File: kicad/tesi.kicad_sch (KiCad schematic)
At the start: 35 parts, among them J1 Conn_01x03_Pin, J2 Conn_01x03_Pin, J3 Conn_01x04_Pin, J4 Conn_01x02_Pin, SW1 POWER, U1 MAX4466, U2 BNO055, U3 MPR121, U4 VL53L1CX

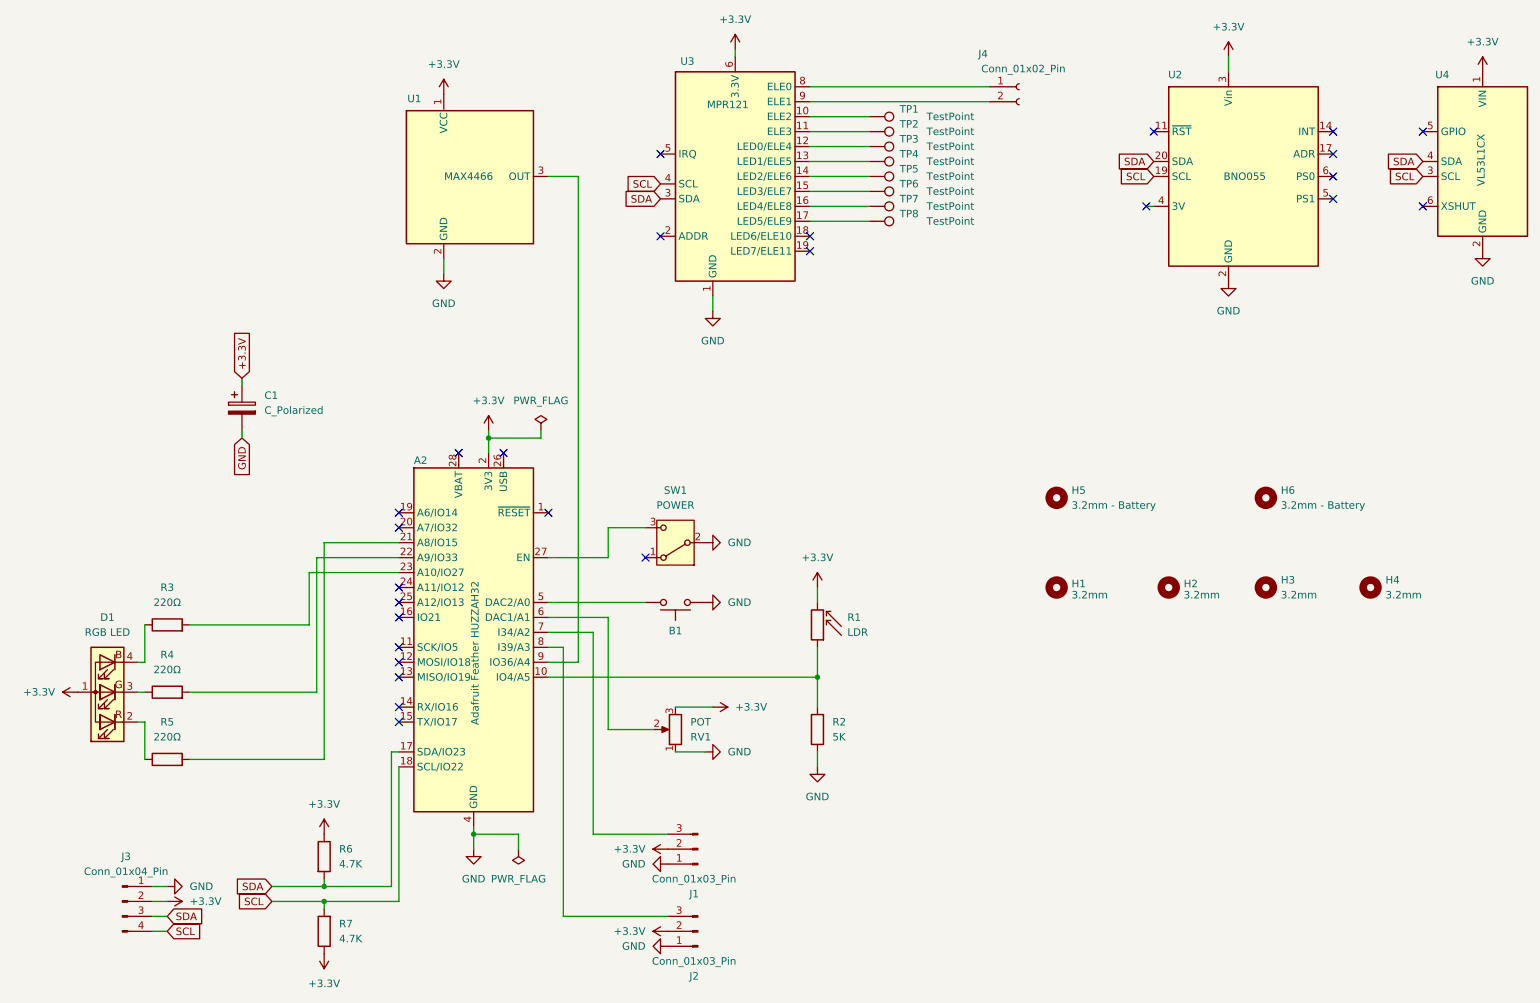
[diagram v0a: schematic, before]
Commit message: updates
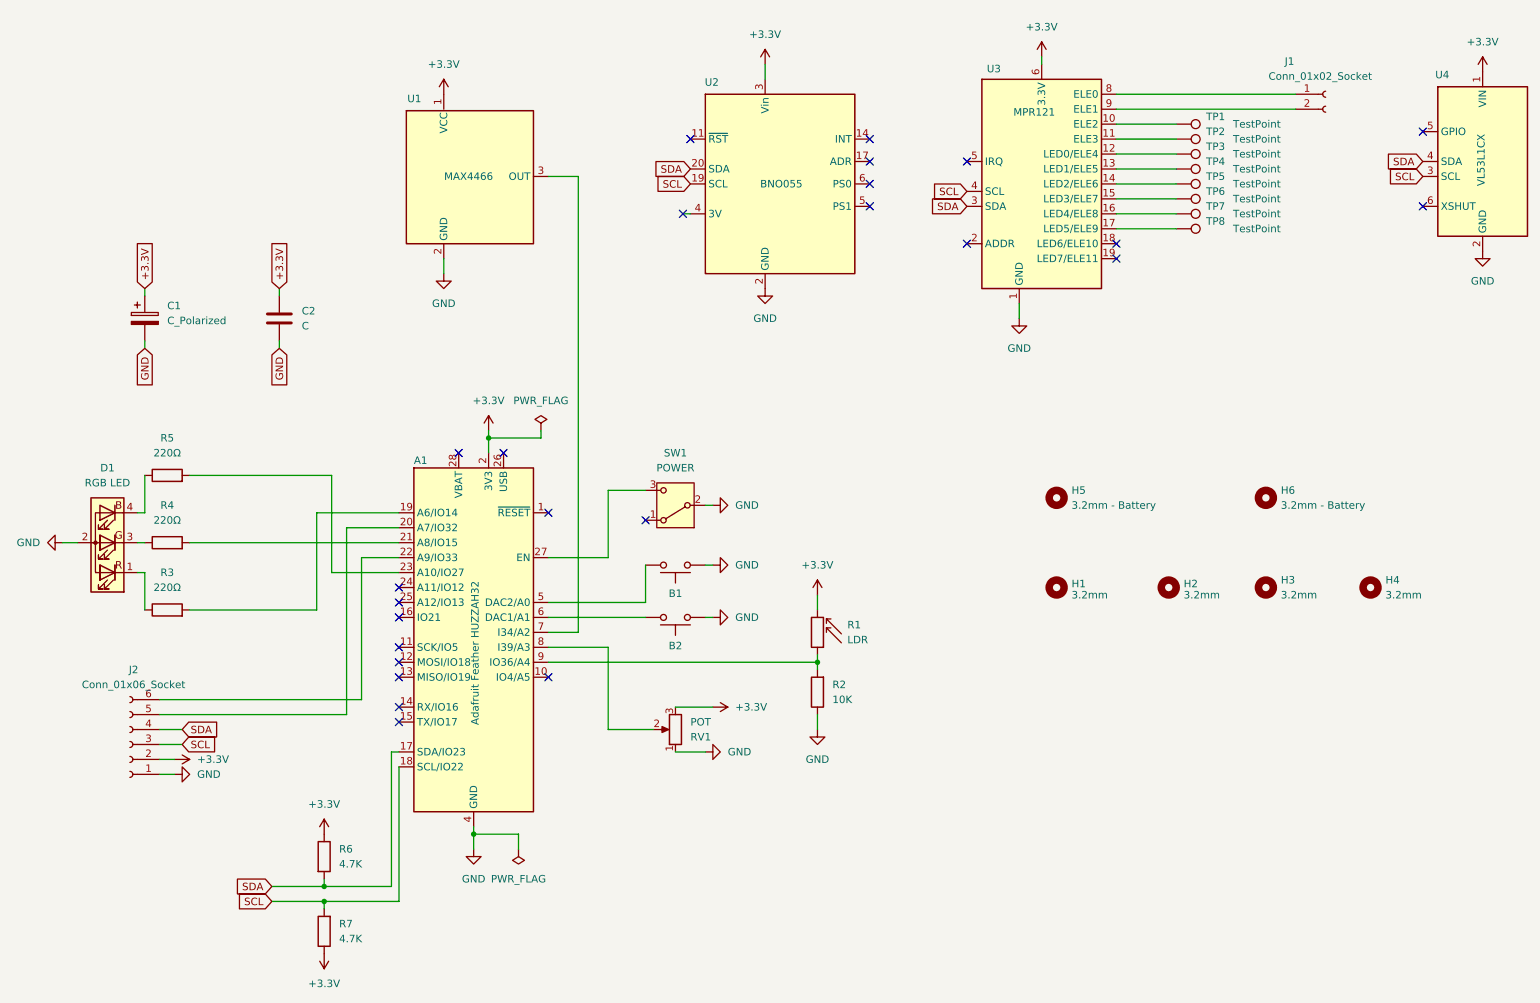
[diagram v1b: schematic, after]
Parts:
- removed J1, J2: Conn_01x03_Pin, Connector_PinSocket_2.54mm:PinSocket_1x03_P2.54mm_Vertical, symbol Connector:Conn_01x03_Pin
- removed J3: Conn_01x04_Pin, Connector_PinSocket_2.54mm:PinSocket_1x04_P2.54mm_Vertical, symbol Connector:Conn_01x04_Pin
- added B2: ~, Button_Switch_THT:SW_PUSH_6mm, symbol Switch:SW_Push
- added C2: C, Capacitor_THT:C_Disc_D4.3mm_W1.9mm_P5.00mm, symbol Device:C
- added J2: Conn_01x06_Socket, Connector_PinSocket_2.54mm:PinSocket_1x06_P2.54mm_Vertical, symbol Connector:Conn_01x06_Socket
- D1: symbol Device:LED_ARGB -> tesi:RGB LED
- J1: renamed from J4; value Conn_01x02_Pin -> Conn_01x02_Socket
- R2: value 5K -> 10K
- renumbered A2 to A1, R5 to R3, R3 to R5
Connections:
- net +3.3V: now also C2.1, J2.2 (Pin_2); no longer D1.1 (A)
- net GND: now also D1.2 (A), B2.1, C2.2, J2.1 (Pin_1)
- net SCL: now also J2.3 (Pin_3)
- net SDA: now also J2.4 (Pin_4)
- net at A1.22 (A9/IO33): now also J2.6 (Pin_6); no longer R4.2
- net at A1.7 (I34/A2): now also U1.3 (OUT)
- net at RV1.2: now also A1.8 (I39/A3); no longer A1.6 (DAC1/A1)
- net at A1.9 (IO36/A4): now also R1.1, R2.2; no longer U1.3 (OUT)
- net at R3.1: now also D1.1 (RK); no longer D1.2 (RK)
- net at A1.21 (A8/IO15): now also R4.2; no longer R3.2
- net at A1.19 (A6/IO14): now also R3.2
- net at A1.20 (A7/IO32): now also J2.5 (Pin_5)
- new net: A1.6 (DAC1/A1), B2.2
- now unconnected: A1.10 (IO4/A5)
- no-connect marks 26 -> 25
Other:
- moved on the sheet: B1, C1, D1, J1, R1, R2, R3, R4, R5, SW1, TP1, TP2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
